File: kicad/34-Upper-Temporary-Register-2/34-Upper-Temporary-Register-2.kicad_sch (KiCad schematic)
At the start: 49 parts

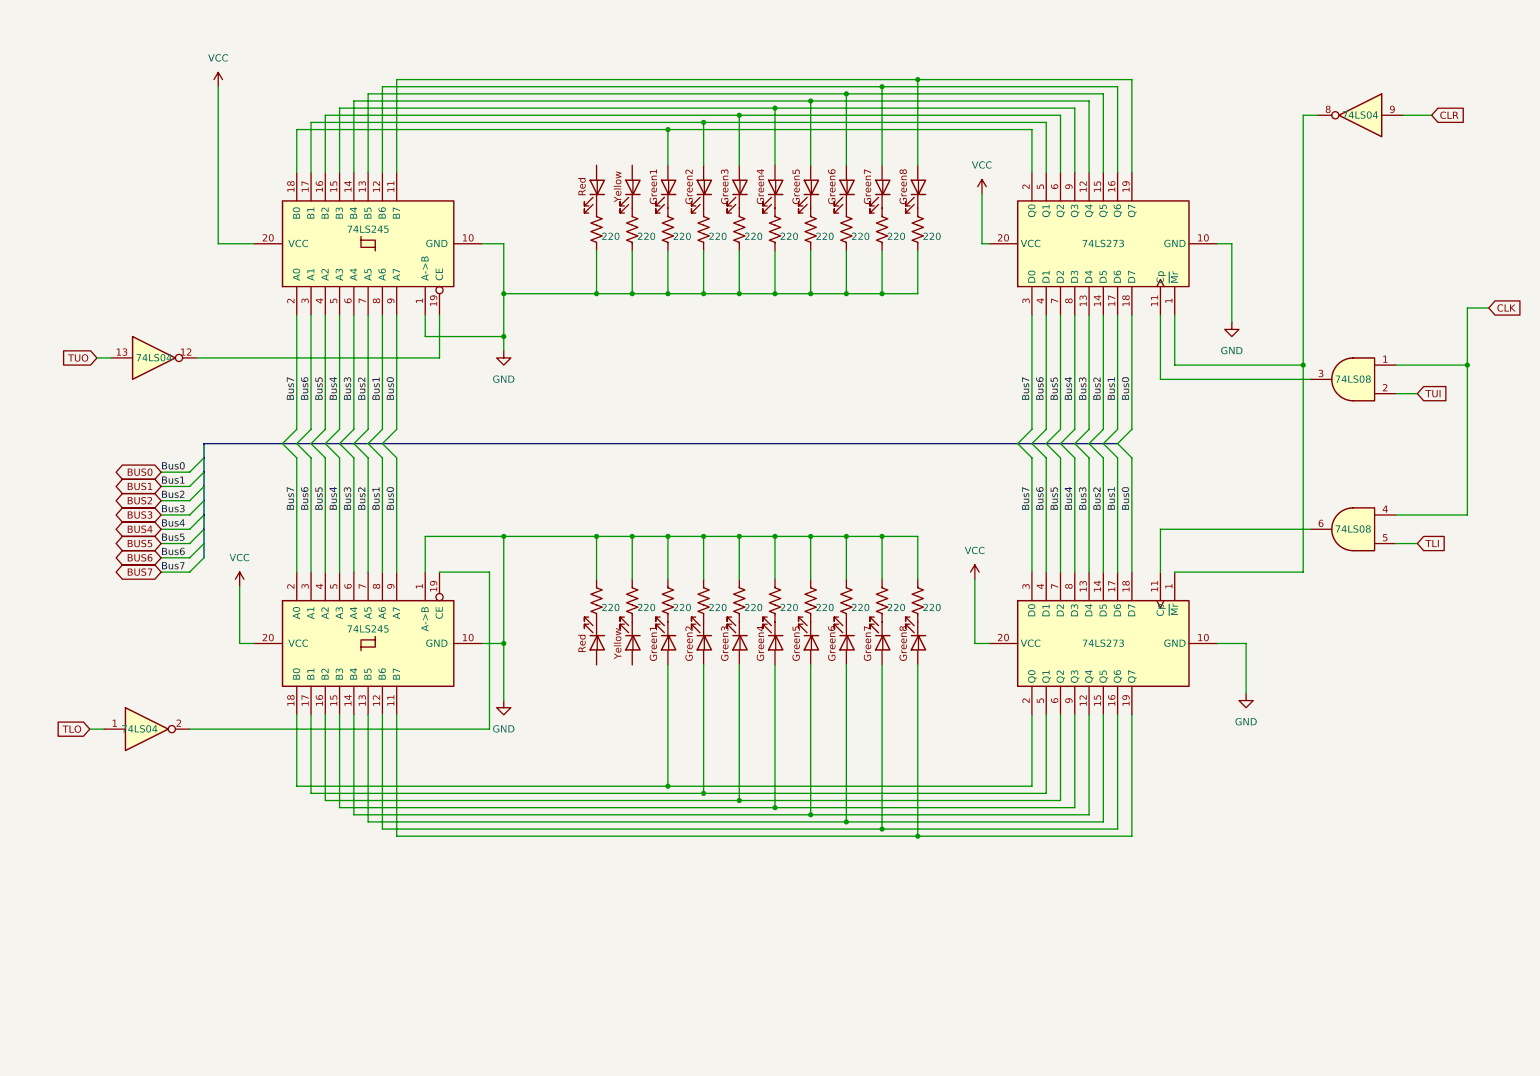
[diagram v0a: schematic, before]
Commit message: Complete the ALU
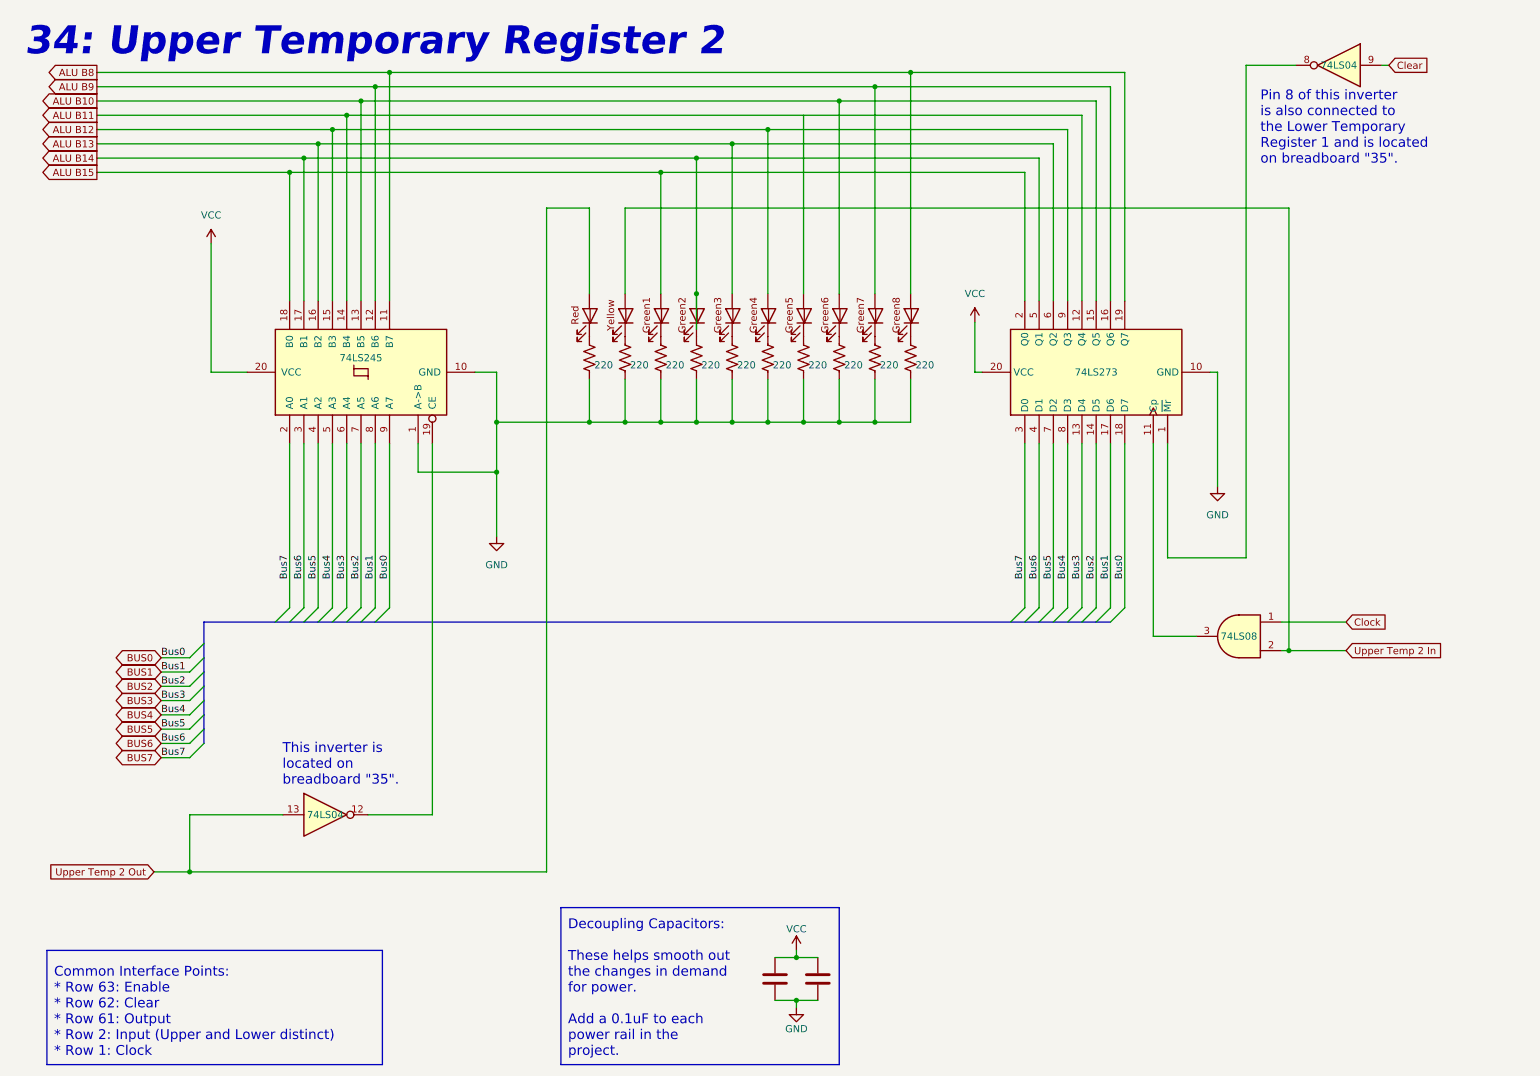
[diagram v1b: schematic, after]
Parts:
- removed R? (x10): 220, symbol Device:R_US
- removed U? (x10): SB1R1Y8G_LED, symbol SB1R1Y8G:SB1R1Y8G_LED
- removed U?: 74LS08, symbol 74xx:74LS08
- removed U?: 74LS04, symbol 74xx:74LS04
- removed U?: 74LS245, symbol 74xx:74LS245
- removed U?: 74LS273, symbol 74xx:74LS273
- added C? (x2): 0.1uF, symbol Device:C
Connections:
- net TUI is gone; now on net Upper Temp 2 In: U?.2
- net TUO is gone; now on net Upper Temp 2 Out: U?.13
- net GND: now also C?.2, C?.2
- net VCC: now also C?.1, C?.1
- net ALU B11: now reaches U?.12 (Q4), U?.14 (B4)
- net ALU B11: no longer U?.17
- net ALU B12: now reaches U?.15 (B3), U?.16, U?.9 (Q3)
- net ALU B8 : now reaches U?.10, U?.11 (B7), U?.19 (Q7)
- net ALU B9 : now reaches U?.12 (B6), U?.16 (Q6), U?.19
- net ALU B10: now reaches U?.13 (B5), U?.15 (Q5), U?.18
- net ALU B13: now reaches U?.15, U?.16 (B2), U?.6 (Q2)
- net ALU B14: now reaches U?.14, U?.17 (B1), U?.5 (Q1)
- net ALU B15: now reaches U?.13, U?.18 (B0), U?.2 (Q0)
- net Upper Temp 2 In: now reaches U?.12
- net Upper Temp 2 Out: now reaches U?.11
- net CLK renamed Clock
- net CLR renamed Clear
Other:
- note added: "34: Upper Temporary Register 2"
- note added: "Common Interface Points: * Row 63: Enable * Row 62: Clear * Row 61: Output * Row 2: Input (Upper and Lower distinct) * Row 1: Clock"
- note added: "Decoupling Capacitors: These helps smooth out the changes in demand for power. Add a 0.1uF to each power rail in the project."
- note added: "Pin 8 of this inverter is also connected to the Lower Temporary Register 1 and is located on breadboard "35"."
- note added: "This inverter is located on breadboard "35"."
- title: (none) -> 34: Upper Temporary Register 2
